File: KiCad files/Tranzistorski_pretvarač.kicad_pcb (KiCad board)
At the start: 2 copper layers, 94.5 x 79.5 mm, 31 parts, among them J1 Screw_Terminal_01x01, J2 Screw_Terminal_01x01, J3 Conn_01x03_Male, J4 Conn_01x01_Male, J5 Screw_Terminal_01x03, J6 Conn_01x01_Male, J7 Conn_01x01_Male, J8 Conn_01x01_Male, Q1 IRLZ44N, U1 SG3524, U2 PC817

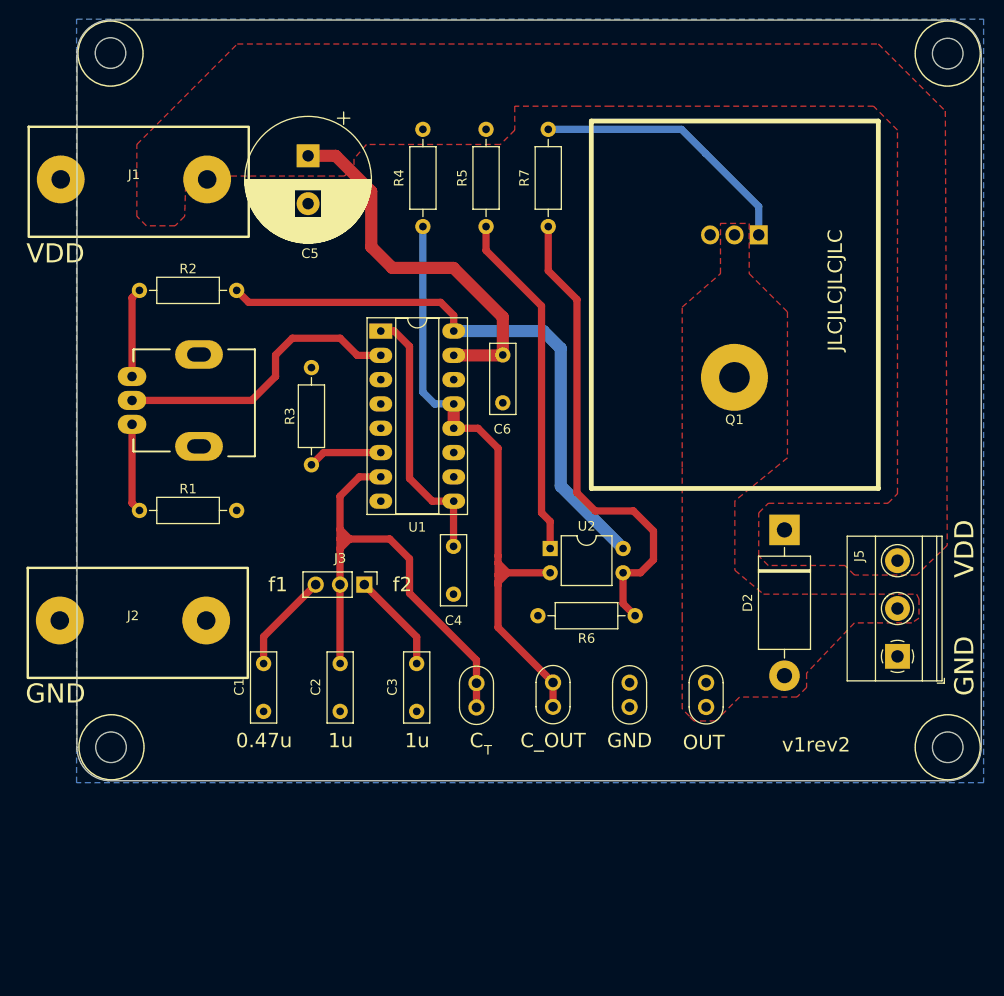
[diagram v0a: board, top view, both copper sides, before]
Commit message: v2
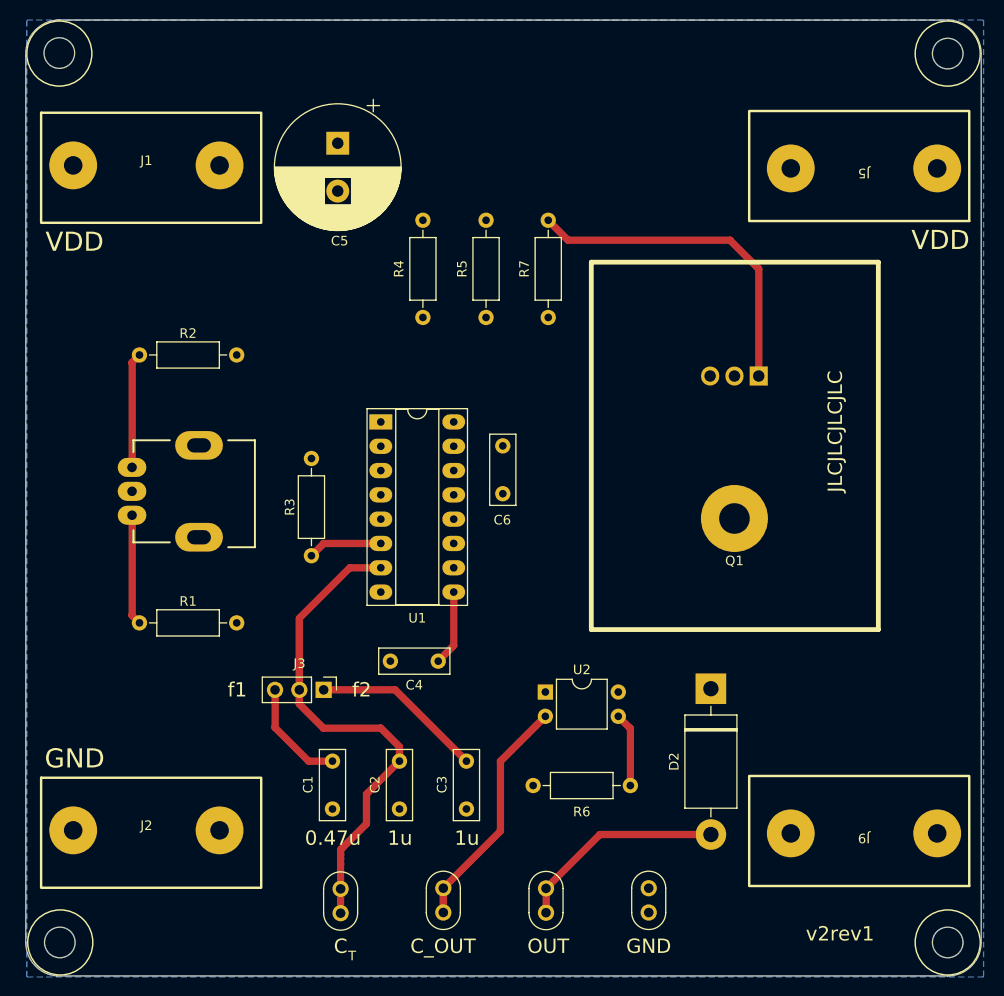
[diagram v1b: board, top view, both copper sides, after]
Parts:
- added J9: Screw_Terminal_01x01, footprint:DELTRON 4mm banana socket - black, F.Cu at (176.5, 139.5)
- J5: value Screw_Terminal_01x03 -> Screw_Terminal_01x01; footprint TerminalBlock_Phoenix:TerminalBlock_Phoenix_MKDS-1,5-3_1x03_P5.00mm_Horizontal -> footprint:DELTRON 4mm banana socket - red
- moved J5 51.1 mm to (176.5, 70.0), turned to 180 degrees
- moved J4 27.2 mm to (143.3, 145.2)
- moved J7 25.8 mm to (121.8, 145.3)
- moved J6 24.4 mm to (132.5, 145.2)
- moved J2 22.0 mm to (101.5, 139.2)
- moved J8 21.6 mm to (154.0, 145.2)
- moved H3 21.1 mm to (92.5, 150.9)
- moved G*** 20.5 mm to (174.5, 149.5)
- moved H1 20.4 mm to (185.2, 150.9)
- moved D2 18.3 mm to (160.5, 124.4)
- moved R6 17.8 mm to (152.1, 134.5)
- moved U2 15.0 mm to (143.2, 124.7)
- moved Q1 14.8 mm to (165.5, 91.7)
- moved C1 12.5 mm to (121.0, 131.9)
- moved C4 12.1 mm to (132.0, 121.5), turned to 180 degrees
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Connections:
- J5 pad 1: GND -> VDD
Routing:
- net /+5V_REF: track 60.9 -> 0.00 mm
- net Net-(R6-Pad1): track 50.5 -> 7.76 mm
- net Net-(J6-Pad1): track 67.1 -> 24.9 mm
- net VDD: track 39.8 -> 0.00 mm
- net Net-(R5-Pad2): track 36.4 -> 0.00 mm
- net Net-(RV1-Pad2): track 30.8 -> 0.00 mm
- net Net-(D2-Pad2): track 0.00 -> 22.1 mm
- net Net-(C4-Pad1): track 27.8 -> 7.89 mm
- net Net-(C3-Pad1): track 10.5 -> 18.0 mm
- net Net-(Q1-Pad1): track 28.3 -> 35.3 mm
- net Net-(R2-Pad2): track 9.32 -> 12.1 mm
- net Net-(R1-Pad1): track 9.32 -> 11.6 mm
- net Net-(C1-Pad1): track 10.5 -> 11.4 mm
- removed copper zone on F.Cu, net Net-(D2-Pad2)
- removed copper zone on F.Cu, net VDD
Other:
- board size 94.5 x 79.5 mm -> 99.9 x 99.9 mm
- board text added: "v2rev1"
- board text removed: "v1rev2"

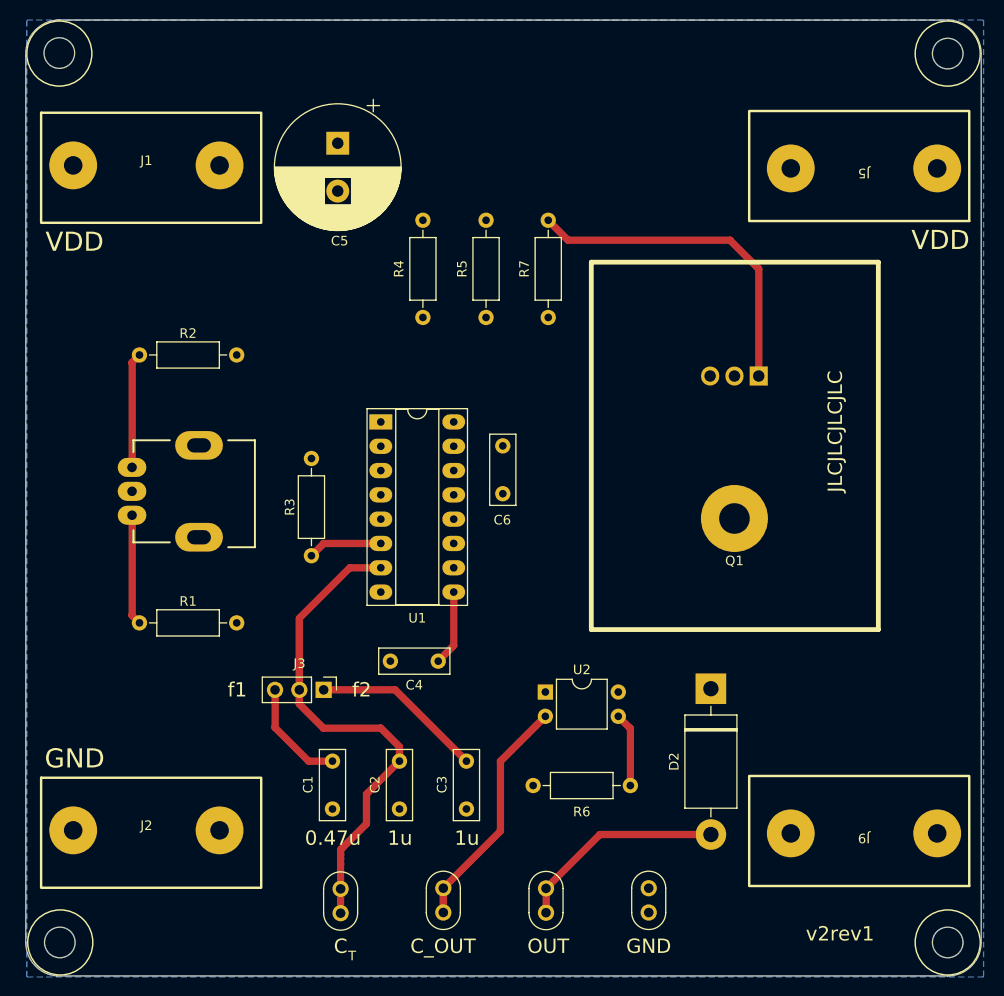
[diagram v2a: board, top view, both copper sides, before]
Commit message: layout
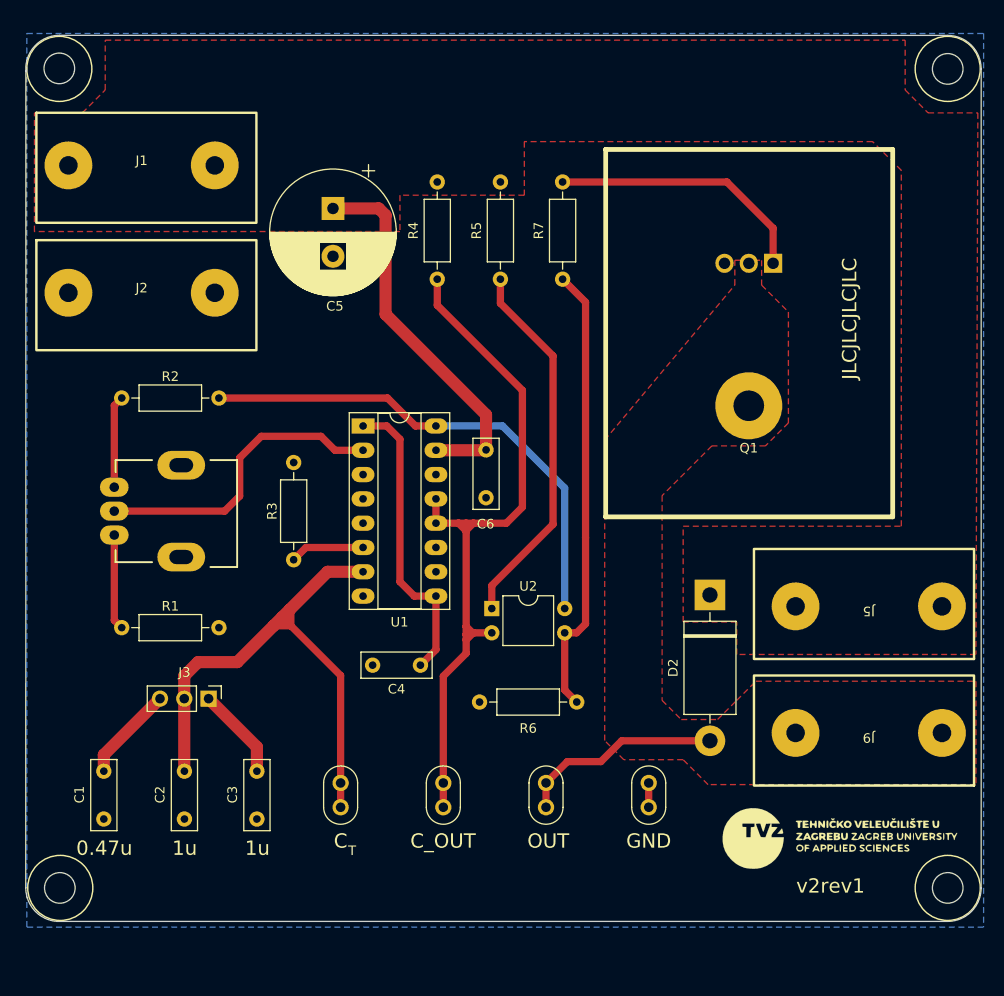
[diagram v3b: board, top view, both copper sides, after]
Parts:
- added G***: LOGO, footprint:tvz, F.Cu at (174.0, 140.0)
- moved J2 56.2 mm to (101.0, 83.0)
- moved J5 45.8 mm to (177.0, 115.8)
- moved C1 23.9 mm to (97.0, 133.0)
- moved C2 22.5 mm to (105.5, 133.0)
- moved C3 21.9 mm to (113.0, 133.0)
- moved J3 12.1 mm to (108.0, 125.4)
- moved Q1 11.9 mm to (167.0, 79.9)
- moved G*** 11.5 mm to (174.5, 138.0)
- moved J7 11.1 mm to (121.8, 134.2)
- moved J4 11.0 mm to (143.3, 134.2)
- moved J6 11.0 mm to (132.5, 134.2)
- moved J8 11.0 mm to (154.0, 134.2)
- moved J9 10.5 mm to (177.0, 129.0)
- moved R6 10.4 mm to (146.5, 125.8)
- moved U2 10.4 mm to (137.6, 116.0)
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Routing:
- net Net-(J6-Pad1): track 24.9 -> 77.7 mm
- net /+5V_REF: track 0.00 -> 52.6 mm
- net VDD: track 0.00 -> 39.9 mm
- net Net-(R6-Pad1): track 7.76 -> 47.3 mm
- net Net-(R5-Pad2): track 0.00 -> 39.3 mm
- net Net-(RV1-Pad2): track 0.00 -> 32.2 mm
- net Net-(C4-Pad1): track 7.89 -> 31.6 mm
- net Net-(C3-Pad1): track 18.0 -> 9.67 mm
- net Net-(Q1-Pad1): track 35.3 -> 27.7 mm
- net /CT: track 51.9 -> 59.1 mm
- net GND: track 0.00 -> 2.54 mm
- net Net-(R2-Pad2): track 12.1 -> 9.64 mm
- net Net-(R1-Pad1): track 11.6 -> 10.0 mm
- net Net-(C1-Pad1): track 11.4 -> 10.0 mm
- net Net-(D2-Pad2): track 22.1 -> 21.5 mm
- added copper zone on F.Cu, net Net-(D2-Pad2)
- added copper zone on F.Cu, net VDD
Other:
- board size 99.9 x 99.9 mm -> 99.9 x 92.6 mm
- board text removed: "VDD"
- board text removed: "f1"
- board text removed: "f2"
